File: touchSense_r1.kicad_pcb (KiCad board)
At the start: 2 copper layers, 20 x 25 mm, 14 parts, among them J1 breakout, J101 Hatched_Fill, J2 GS2, J3 GS2, J4 cap/daisy, U1 AT42QT1010-TSHR

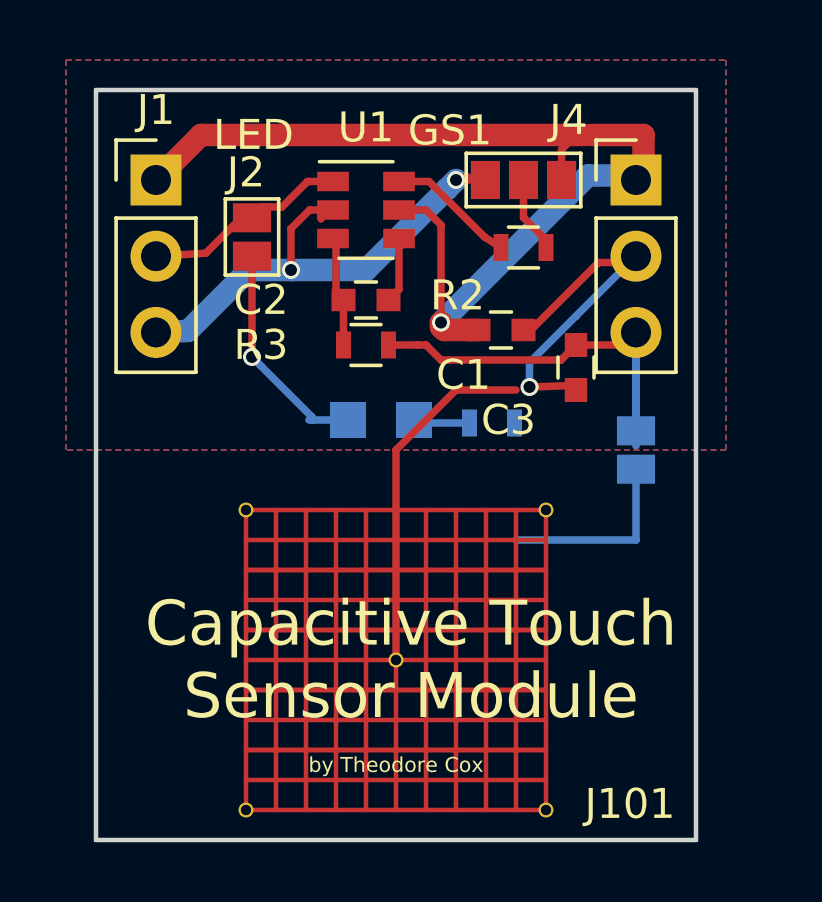
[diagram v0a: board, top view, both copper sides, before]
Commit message: organize project folder, small pcb maitenance, generated gerbers
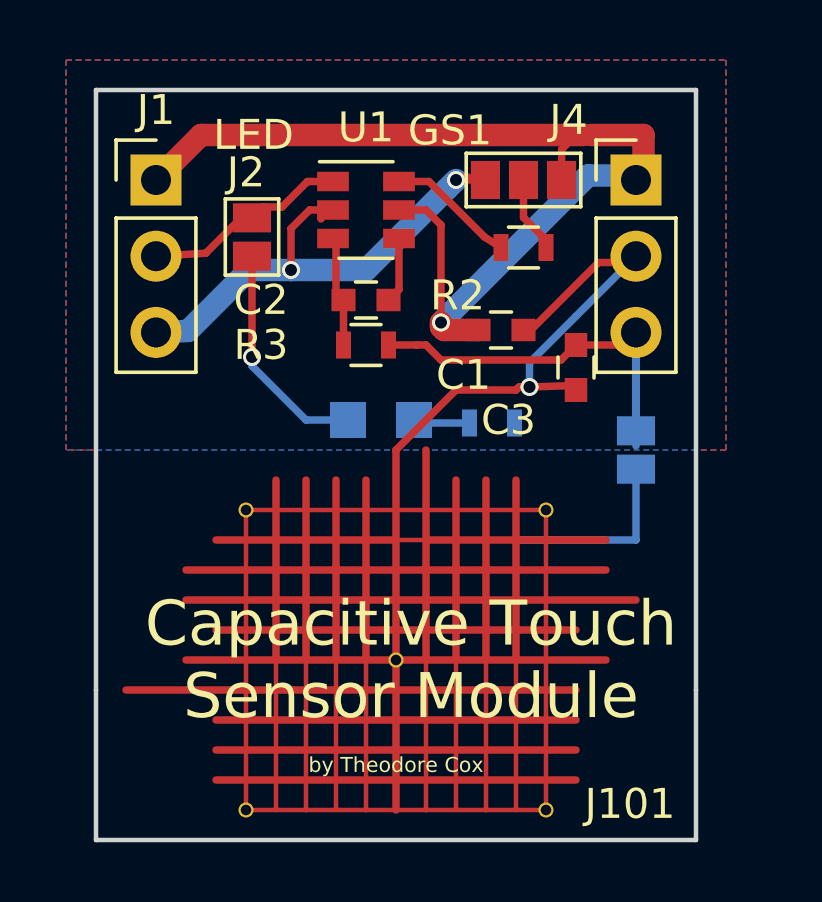
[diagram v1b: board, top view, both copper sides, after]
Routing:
- net GND: track 41.3 -> 213.8 mm
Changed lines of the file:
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@@
     (thickness 1.6)
     (drawings 11)
-    (tracks 99)
+    (tracks 144)
     (zones 0)
     (modules 14)
@@
     (user_trace_width 0.75)
     (trace_clearance 0.2)
-    (zone_clearance 0.381)
+    (zone_clearance 0.3)
     (zone_45_only yes)
     (trace_min 0.2)
@@
     (effects (font (size 0.75 0.75) (thickness 0.1875)) (justify right mirror))
   )
+  (segment (start 113 123) (end 119 123) (width 0.25) (layer F.Cu) (net 1))
+  (segment (start 113 122) (end 119 122) (width 0.25) (layer F.Cu) (net 1))
+  (segment (start 113 123) (end 107 123) (width 0.25) (layer F.Cu) (net 1))
+  (segment (start 113 122) (end 107 122) (width 0.25) (layer F.Cu) (net 1))
+  (segment (start 113 121) (end 107 121) (width 0.25) (layer F.Cu) (net 1))
+  (segment (start 113 121) (end 119 121) (width 0.25) (layer F.Cu) (net 1))
+  (segment (start 117.45 109.9) (end 117.1 109.9) (width 0.25) (layer F.Cu) (net 1))
+  (segment (start 115 110) (end 113 112) (width 0.25) (layer F.Cu) (net 1))
+  (segment (start 113 112) (end 113 115) (width 0.25) (layer F.Cu) (net 1))
   (segment (start 117 110) (end 115 110) (width 0.25) (layer F.Cu) (net 1))
-  (segment (start 113 112) (end 113 119) (width 0.25) (layer F.Cu) (net 1) (status 800000))
-  (segment (start 115 110) (end 113 112) (width 0.25) (layer F.Cu) (net 1))
+  (segment (start 117.1 109.9) (end 117 110) (width 0.25) (layer F.Cu) (net 1))
+  (segment (start 113 120) (end 104 120) (width 0.25) (layer F.Cu) (net 1))
+  (segment (start 113 120) (end 119 120) (width 0.25) (layer F.Cu) (net 1))
+  (segment (start 113 119) (end 113 120) (width 0.25) (layer F.Cu) (net 1))
+  (segment (start 113 120) (end 113 121) (width 0.25) (layer F.Cu) (net 1))
+  (segment (start 113 121) (end 113 122) (width 0.25) (layer F.Cu) (net 1))
+  (segment (start 113 122) (end 113 123) (width 0.25) (layer F.Cu) (net 1))
+  (segment (start 113 123) (end 113 124) (width 0.25) (layer F.Cu) (net 1))
+  (segment (start 114 115) (end 120 115) (width 0.25) (layer F.Cu) (net 1))
+  (segment (start 109 119) (end 109 113) (width 0.25) (layer F.Cu) (net 1))
+  (segment (start 110 119) (end 110 113) (width 0.25) (layer F.Cu) (net 1))
+  (segment (start 111 119) (end 111 113) (width 0.25) (layer F.Cu) (net 1))
+  (segment (start 112 119) (end 112 113) (width 0.25) (layer F.Cu) (net 1))
+  (segment (start 113 115) (end 107 115) (width 0.25) (layer F.Cu) (net 1))
+  (segment (start 113 118) (end 107 118) (width 0.25) (layer F.Cu) (net 1))
+  (segment (start 113 118) (end 119 118) (width 0.25) (layer F.Cu) (net 1))
+  (segment (start 117 119) (end 117 113) (width 0.25) (layer F.Cu) (net 1))
+  (segment (start 116 119) (end 116 113) (width 0.25) (layer F.Cu) (net 1))
+  (segment (start 115 119) (end 115 113) (width 0.25) (layer F.Cu) (net 1))
+  (segment (start 114 119) (end 114 115) (width 0.25) (layer F.Cu) (net 1))
+  (segment (start 114 115) (end 114 112) (width 0.25) (layer F.Cu) (net 1))
+  (segment (start 113 117) (end 121 117) (width 0.25) (layer F.Cu) (net 1))
+  (segment (start 113 116) (end 120 116) (width 0.25) (layer F.Cu) (net 1))
+  (segment (start 113 117) (end 106 117) (width 0.25) (layer F.Cu) (net 1))
+  (segment (start 113 116) (end 106 116) (width 0.25) (layer F.Cu) (net 1))
+  (segment (start 113 119) (end 112 119) (width 0.25) (layer F.Cu) (net 1))
+  (segment (start 112 119) (end 111 119) (width 0.25) (layer F.Cu) (net 1))
+  (segment (start 111 119) (end 110 119) (width 0.25) (layer F.Cu) (net 1))
+  (segment (start 110 119) (end 109 119) (width 0.25) (layer F.Cu) (net 1))
+  (segment (start 109 119) (end 106 119) (width 0.25) (layer F.Cu) (net 1))
+  (segment (start 113 119) (end 114 119) (width 0.25) (layer F.Cu) (net 1))
+  (segment (start 114 119) (end 115 119) (width 0.25) (layer F.Cu) (net 1))
+  (segment (start 115 119) (end 116 119) (width 0.25) (layer F.Cu) (net 1))
+  (segment (start 116 119) (end 117 119) (width 0.25) (layer F.Cu) (net 1))
+  (segment (start 117 119) (end 120 119) (width 0.25) (layer F.Cu) (net 1))
+  (segment (start 113 115) (end 113 116) (width 0.25) (layer F.Cu) (net 1))
+  (segment (start 113 116) (end 113 117) (width 0.25) (layer F.Cu) (net 1))
+  (segment (start 113 117) (end 113 118) (width 0.25) (layer F.Cu) (net 1))
+  (segment (start 113 118) (end 113 119) (width 0.25) (layer F.Cu) (net 1))
   (segment (start 112 106) (end 114.700001 103.299999) (width 0.75) (layer B.Cu) (net 1))
   (segment (start 109.5 106) (end 112 106) (width 0.75) (layer B.Cu) (net 1))
@@
   (segment (start 111 105.05) (end 110.9 104.95) (width 0.25) (layer F.Cu) (net 7) (status 30))
   (segment (start 111.25 108.5) (end 111.25 107) (width 0.25) (layer F.Cu) (net 7) (status 10))
-  (segment (start 108.499999 109.199999) (end 108.2 108.9) (width 0.25) (layer B.Cu) (net 8))
-  (segment (start 110.2 111) (end 110.2 110.9) (width 0.25) (layer B.Cu) (net 8))
+  (segment (start 108.2 108.9) (end 108.2 109.2) (width 0.25) (layer B.Cu) (net 8))
+  (via (at 108.2 108.9) (size 0.6) (drill 0.4) (layers F.Cu B.Cu) (net 8))
   (segment (start 108.2 105.54) (end 108.2 108.9) (width 0.25) (layer F.Cu) (net 8))
-  (segment (start 110.2 110.9) (end 108.499999 109.199999) (width 0.25) (layer B.Cu) (net 8))
-  (via (at 108.2 108.9) (size 0.6) (drill 0.4) (layers F.Cu B.Cu) (net 8))
+  (segment (start 110 111) (end 111.4 111) (width 0.25) (layer B.Cu) (net 8) (status 800000))
+  (segment (start 108.2 109.2) (end 110 111) (width 0.25) (layer B.Cu) (net 8))
+  (segment (start 111.25 110.85) (end 111.4 111) (width 0.25) (layer B.Cu) (net 8))
   (segment (start 108.56 105.54) (end 108.2 105.54) (width 0.25) (layer F.Cu) (net 8) (status 30))
-  (segment (start 110.1 111) (end 110.2 111) (width 0.25) (layer B.Cu) (net 8))
-  (segment (start 110.2 111) (end 111.75 111) (width 0.25) (layer B.Cu) (net 8))
   (segment (start 115.45 111.1) (end 113.7 111.1) (width 0.25) (layer B.Cu) (net 9))
   (segment (start 113.7 111.1) (end 113.6 111) (width 0.25) (layer B.Cu) (net 9))
@@
     (polygon
       (pts
-        (xy 124 112) (xy 102 112) (xy 102 99) (xy 124 99)
+        (xy 124 112) (xy 123 112) (xy 123 125) (xy 103 125) (xy 103 112)
+        (xy 102 112) (xy 102 99) (xy 124 99)
       )
     )
